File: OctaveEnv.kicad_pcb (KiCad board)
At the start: 4 copper layers, 89 parts, among them J101 IN, J102 PWR, J103 OUT, Q101 BC857, SW101 Stomp, U101 AZ34063U, U102 L7805, U103 TL074, U104 74HCT74, U105 LM13700, U106 TL074, U107 TL072

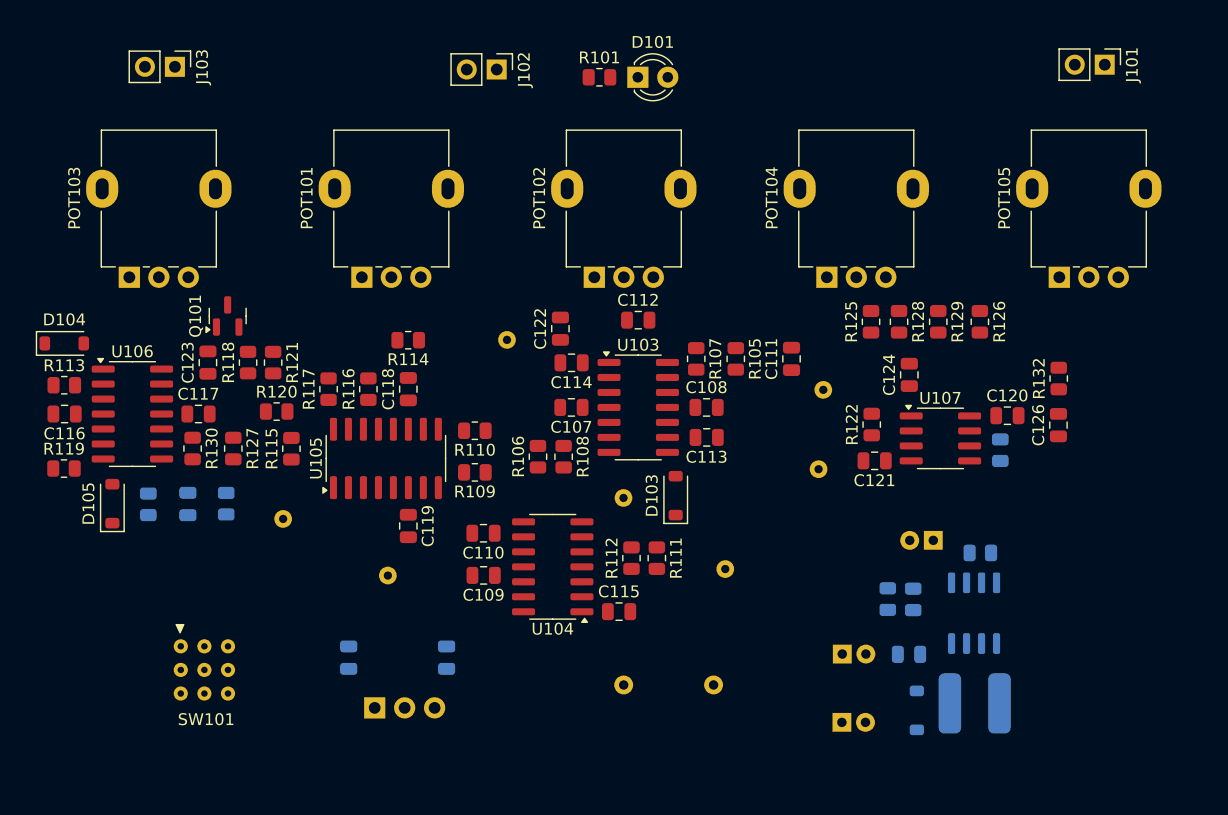
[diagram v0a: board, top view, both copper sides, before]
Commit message: silkscreen stuff, new layout
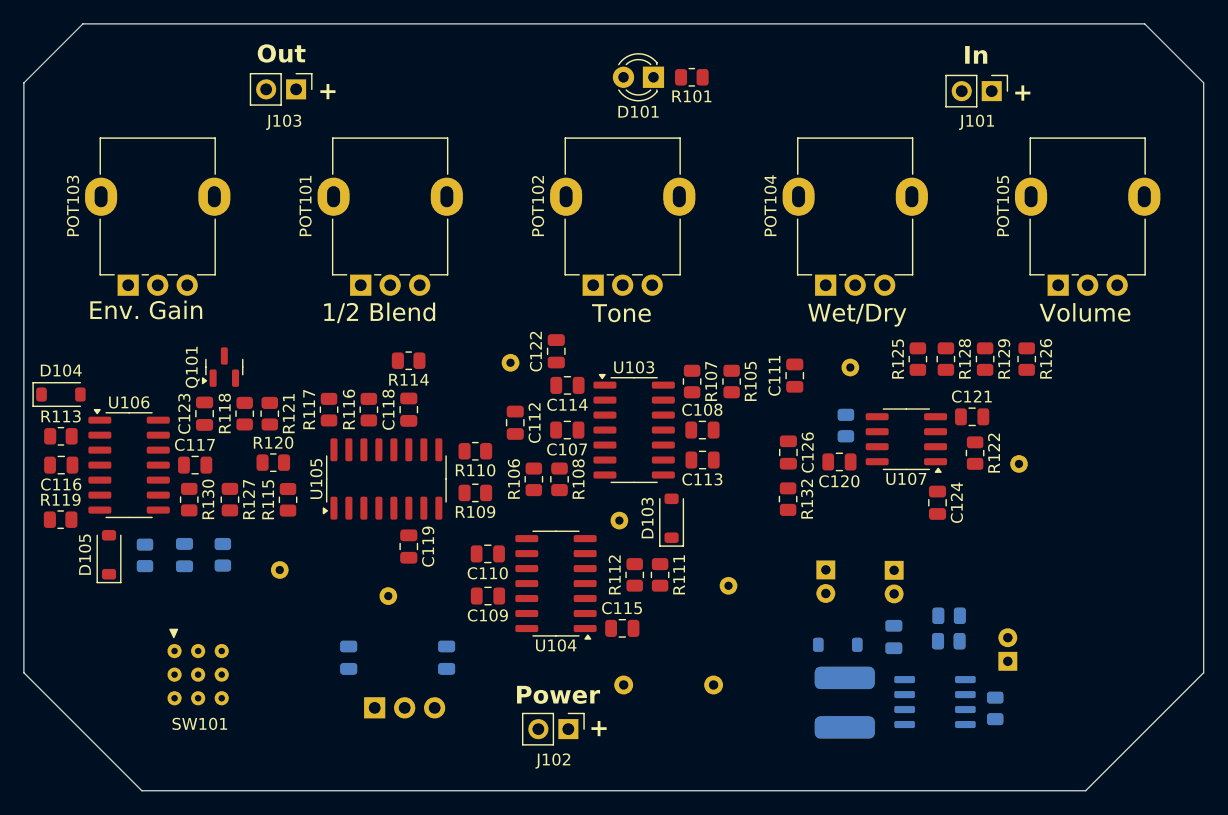
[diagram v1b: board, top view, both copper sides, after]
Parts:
- moved J102 56.2 mm to (46.1, 59.8)
- moved R132 25.1 mm to (64.8, 40.3), turned to -90 degrees
- moved C126 23.0 mm to (64.8, 36.3), turned to -90 degrees
- moved TP104 17.7 mm to (84.3, 37.3), turned to -90 degrees
- moved C120 14.8 mm to (69.1, 37.1), turned to 180 degrees
- moved C112 13.6 mm to (41.6, 33.8), turned to -90 degrees
- moved R131 13.3 mm to (69.7, 34.0), turned to -90 degrees
- moved R102 13.2 mm to (82.3, 58.0), turned to -90 degrees
- moved C106 13.0 mm to (68.0, 46.3), turned to -90 degrees
- moved C101 12.0 mm to (83.4, 54.0), turned to 90 degrees
- moved C124 11.1 mm to (77.4, 40.6), turned to -90 degrees
- moved L101 11.0 mm to (69.6, 57.5), turned to 90 degrees
- moved J103 10.5 mm to (23.1, 5.55)
- moved J101 9.84 mm to (82.0, 5.70)
- moved R122 9.09 mm to (80.6, 36.4), turned to -90 degrees
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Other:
- board outline added: 100 x 65 mm
- board text added: "+"
- board text added: "1/2 Blend"
- board text added: "Env. Gain"
- board text added: "In"
- board text added: "Out"
- board text added: "Power"
- board text added: "Tone"
- board text added: "Volume"
- board text added: "Wet/Dry"
